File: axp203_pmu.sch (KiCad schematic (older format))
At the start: 1 part, among them U1 AXP203

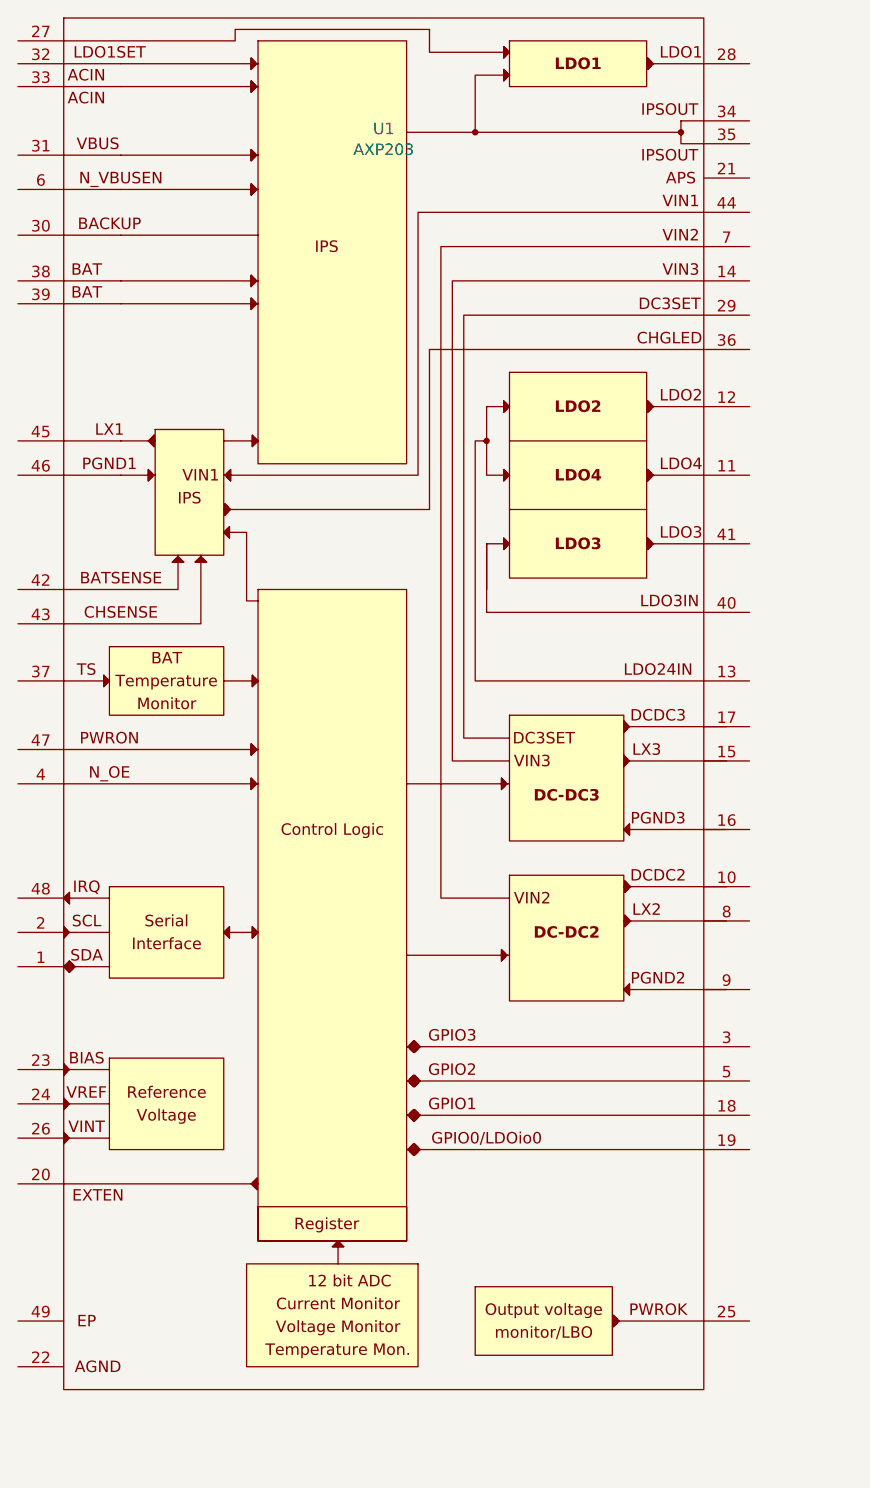
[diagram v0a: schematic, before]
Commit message: Continue activity
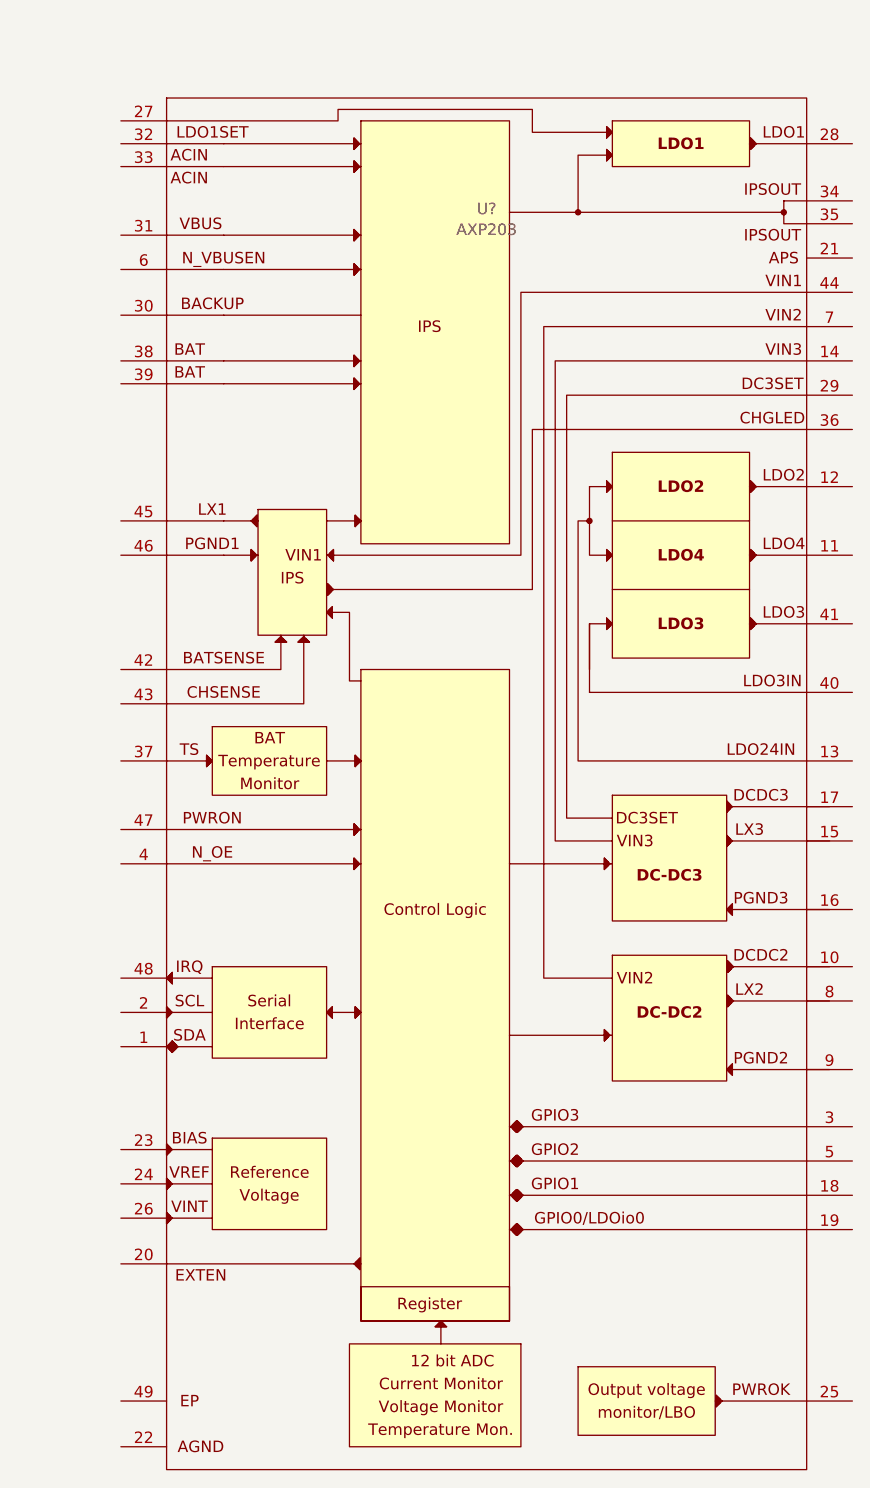
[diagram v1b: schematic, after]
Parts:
- removed U1: AXP203, X_Powers:AXP203_QFN48, symbol x_powers:AXP203
- added U?: AXP203, symbol x_powers:AXP203
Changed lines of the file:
@@
 $EndDescr
 $Comp
-L x_powers:AXP203 U1
-U 1 1 5E09CC8E
-P 7900 5000
-F 0 "U1" H 7900 7565 50  0000 C CNN
-F 1 "AXP203" H 7900 7474 50  0000 C CNN
-F 2 "X_Powers:AXP203_QFN48" H 3550 7200 50  0001 C CNN
-F 3 "/home/mw/kicad_library/Schematic/PMU_Units/X_Powers/Components_Documentation/AXP203_Datasheet_V1.0.pdf" H 3550 7200 50  0001 C CNN
-	1    7900 5000
+L x_powers:AXP203 U?
+U 1 1 5E04BBCA
+P 8350 5350
+F 0 "U?" H 8350 7915 50  0000 C CNN
+F 1 "AXP203" H 8350 7824 50  0000 C CNN
+F 2 "" H 4000 7550 50  0001 C CNN
+F 3 "/home/mw/kicad_library/Schematic/PMU_Units/X_Powers/Components_Documentation/AXP203_Datasheet_V1.0.pdf" H 4000 7550 50  0001 C CNN
+	1    8350 5350
 	1    0    0    -1
 $EndComp
